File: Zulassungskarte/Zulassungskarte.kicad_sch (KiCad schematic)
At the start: 40 parts, among them J1 Conn_02x04_Counter_Clockwise, J2 Conn_02x04_Counter_Clockwise, J3 Conn_01x04_Pin, J4 Conn_02x03_Odd_Even, U1 ATmega48

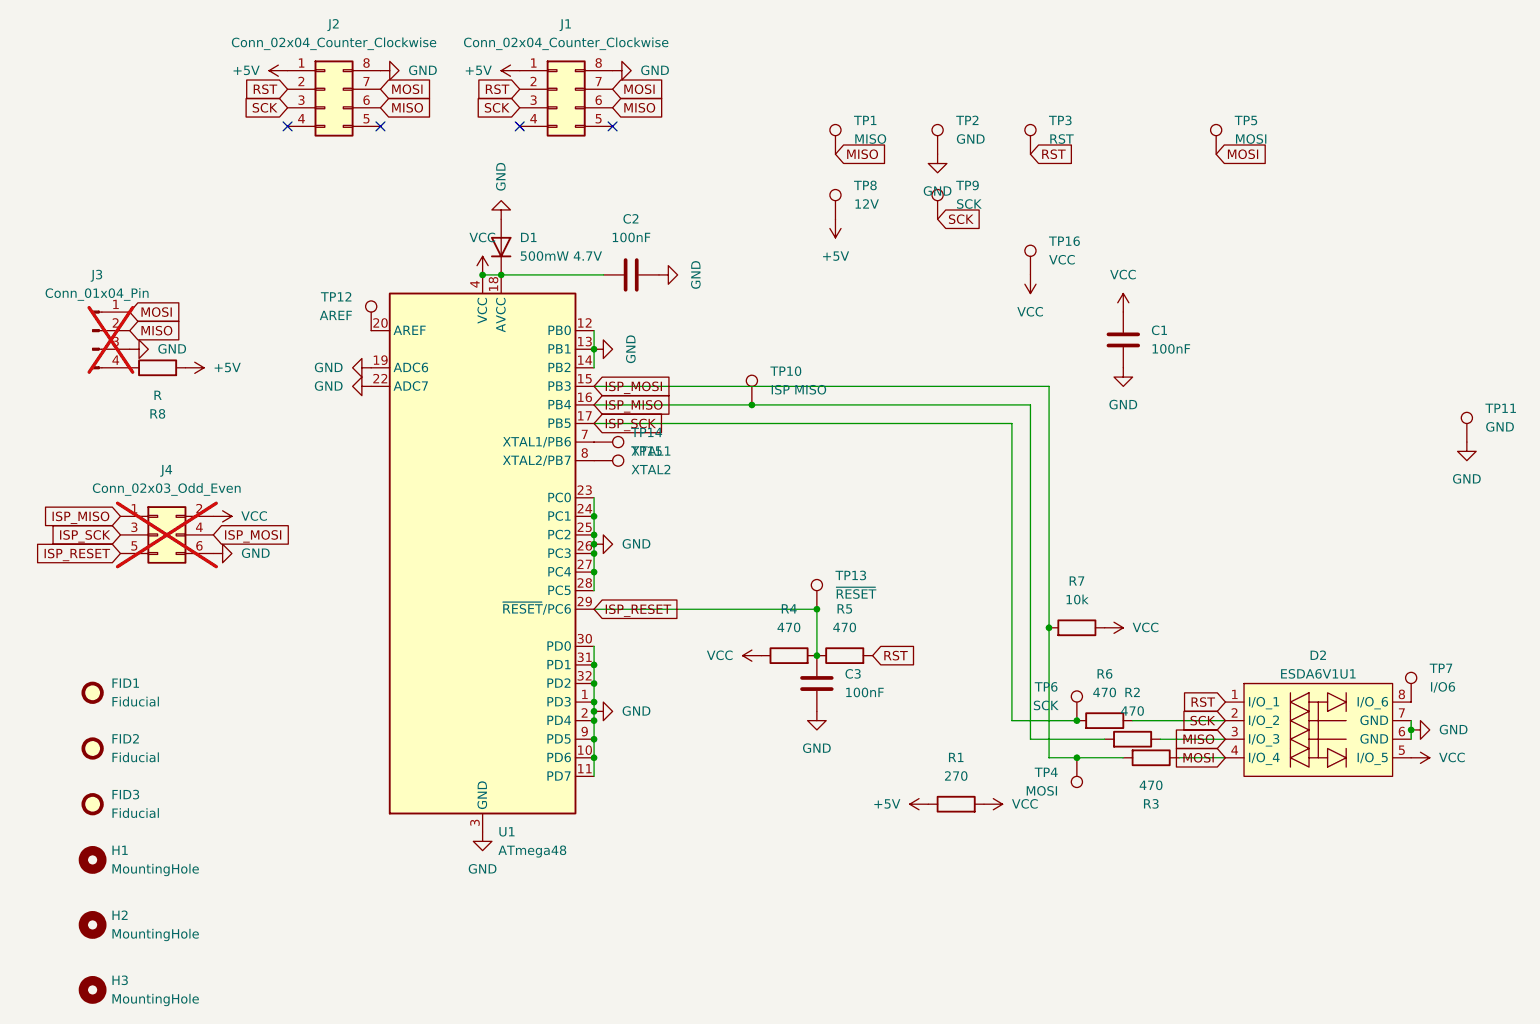
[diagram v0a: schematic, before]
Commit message: 12v zlk
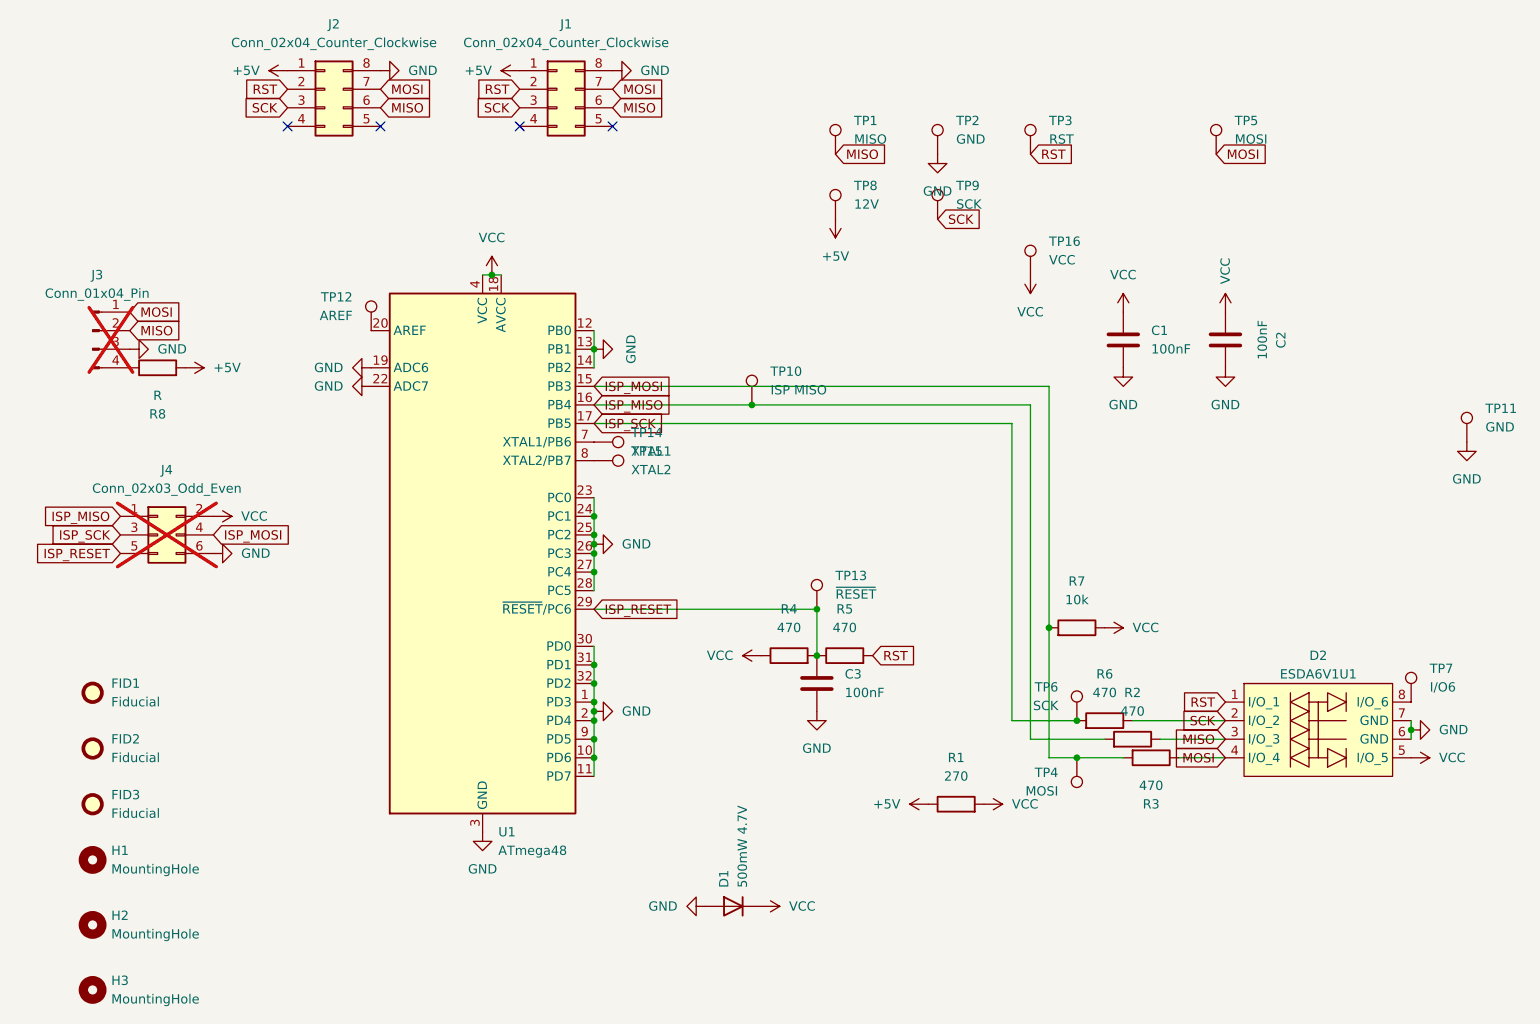
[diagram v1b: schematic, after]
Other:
- moved on the sheet: C2, D1
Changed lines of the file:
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@@
 	)
 	(junction
-		(at 72.39 49.53)
-		(diameter 0)
-		(color 0 0 0 0)
-	)
-	(junction
 		(at 87.63 59.69)
 		(diameter 0)
@@
 	)
 	(junction
-		(at 74.93 49.53)
+		(at 87.63 105.41)
 		(diameter 0)
 		(color 0 0 0 0)
 	)
 	(junction
-		(at 87.63 105.41)
+		(at 87.63 109.22)
 		(diameter 0)
 		(color 0 0 0 0)
 	)
 	(junction
-		(at 87.63 109.22)
+		(at 73.66 49.53)
 		(diameter 0)
 		(color 0 0 0 0)
@@
 	(wire
 		(pts
-			(xy 72.39 49.53) (xy 74.93 49.53)
-		)
-		(stroke
-			(width 0)
-			(type default)
-		)
-	)
-	(wire
-		(pts
 			(xy 157.48 113.03) (xy 147.32 113.03)
 		)
@@
 	(wire
 		(pts
-			(xy 87.63 100.33) (xy 87.63 102.87)
+			(xy 73.66 49.53) (xy 74.93 49.53)
 		)
 		(stroke
@@
 	(wire
 		(pts
-			(xy 87.63 90.17) (xy 87.63 92.71)
+			(xy 87.63 100.33) (xy 87.63 102.87)
 		)
 		(stroke
@@
 	(wire
 		(pts
-			(xy 74.93 49.53) (xy 88.9 49.53)
+			(xy 87.63 90.17) (xy 87.63 92.71)
 		)
 		(stroke
@@
 	(wire
 		(pts
+			(xy 73.66 49.53) (xy 72.39 49.53)
+		)
+		(stroke
+			(width 0)
+			(type default)
+		)
+	)
+	(wire
+		(pts
 			(xy 87.63 107.95) (xy 87.63 105.41)
 		)
@@
 	(symbol
 		(lib_id "power:GND")
-		(at 74.93 41.91 0)
+		(at 102.87 135.89 270)
 		(mirror x)
 		(unit 1)
@@
 		(fields_autoplaced yes)
 		(property "Reference" "#PWR024"
-			(at 74.93 35.56 0)
+			(at 96.52 135.89 0)
 			(effects
 				(font
@@
 		)
 		(property "Value" "GND"
-			(at 74.9301 38.1 90)
+			(at 99.06 135.8899 90)
 			(effects
 				(font
@@
 		)
 		(property "Footprint" ""
-			(at 74.93 41.91 0)
+			(at 102.87 135.89 0)
 			(effects
 				(font
@@
 		)
 		(property "Datasheet" ""
-			(at 74.93 41.91 0)
+			(at 102.87 135.89 0)
 			(effects
 				(font
@@
 		)
 		(property "Description" "Power symbol creates a global label with name \"GND\" , ground"
-			(at 74.93 41.91 0)
+			(at 102.87 135.89 0)
 			(effects
 				(font
@@
 	(symbol
 		(lib_id "power:VCC")
-		(at 72.39 49.53 0)
+		(at 73.66 49.53 0)
 		(unit 1)
 		(exclude_from_sim no)
@@
 		(fields_autoplaced yes)
 		(property "Reference" "#PWR03"
-			(at 72.39 53.34 0)
+			(at 73.66 53.34 0)
 			(effects
 				(font
@@
 		)
 		(property "Value" "VCC"
-			(at 72.39 44.45 0)
+			(at 73.66 44.45 0)
 			(effects
 				(font
@@
 		)
 		(property "Footprint" ""
-			(at 72.39 49.53 0)
+			(at 73.66 49.53 0)
 			(effects
 				(font
@@
 		)
 		(property "Datasheet" ""
-			(at 72.39 49.53 0)
+			(at 73.66 49.53 0)
 			(effects
 				(font
@@
 		)
 		(property "Description" "Power symbol creates a global label with name \"VCC\""
-			(at 72.39 49.53 0)
+			(at 73.66 49.53 0)
 			(effects
 				(font
@@
 	)
 	(symbol
+		(lib_id "power:VCC")
+		(at 110.49 135.89 270)
+		(unit 1)
+		(exclude_from_sim no)
+		(in_bom yes)
+		(on_board yes)
+		(dnp no)
+		(fields_autoplaced yes)
+		(property "Reference" "#PWR08"
+			(at 106.68 135.89 0)
+			(effects
+				(font
+					(size 1.27 1.27)
+				)
+				(hide yes)
+			)
+		)
+		(property "Value" "VCC"
+			(at 114.3 135.8899 90)
+			(effects
+				(font
+					(size 1.27 1.27)
+				)
+				(justify left)
+			)
+		)
+		(property "Footprint" ""
+			(at 110.49 135.89 0)
+			(effects
+				(font
+					(size 1.27 1.27)
+				)
+				(hide yes)
+			)
+		)
+		(property "Datasheet" ""
+			(at 110.49 135.89 0)
+			(effects
+				(font
+					(size 1.27 1.27)
+				)
+				(hide yes)
+			)
+		)
+		(property "Description" "Power symbol creates a global label with name \"VCC\""
+			(at 110.49 135.89 0)
+			(effects
+				(font
+					(size 1.27 1.27)
+				)
+				(hide yes)
+			)
+		)
+		(pin "1"
+		)
+		(instances
+			(project "Zulassungskarte"
+				(path "/f437cf05-d297-460e-8639-991b777c08ac"
+					(reference "#PWR08")
+					(unit 1)
+				)
+			)
+		)
+	)
+	(symbol
 		(lib_id "power:GND")
 		(at 199.39 111.76 90)
@@
 	(symbol
 		(lib_id "Device:D")
-		(at 74.93 45.72 270)
-		(mirror x)
+		(at 106.68 135.89 0)
+		(mirror y)
 		(unit 1)
 		(exclude_from_sim no)
@@
 		(fields_autoplaced yes)
 		(property "Reference" "D1"
-			(at 77.47 44.4499 90)
+			(at 105.4099 133.35 90)
 			(effects
 				(font
@@
 		)
 		(property "Value" "500mW 4.7V"
-			(at 77.47 46.9899 90)
+			(at 107.9499 133.35 90)
 			(effects
 				(font
@@
 		)
 		(property "Footprint" "Diode_SMD:D_SOD-123"
-			(at 74.93 45.72 0)
+			(at 106.68 135.89 0)
 			(effects
 				(font
@@
 		)
 		(property "Datasheet" "~"
-			(at 74.93 45.72 0)
+			(at 106.68 135.89 0)
 			(effects
 				(font
@@
 		)
 		(property "Description" "Diode"
-			(at 74.93 45.72 0)
+			(at 106.68 135.89 0)
 			(effects
 				(font
@@
 		)
 		(property "Sim.Device" "D"
-			(at 74.93 45.72 0)
+			(at 106.68 135.89 0)
 			(effects
 				(font
@@
 		)
 		(property "Sim.Pins" "1=K 2=A"
-			(at 74.93 45.72 0)
+			(at 106.68 135.89 0)
 			(effects
 				(font
@@
 	(symbol
 		(lib_id "Device:C")
-		(at 92.71 49.53 90)
+		(at 173.99 58.42 0)
 		(unit 1)
 		(exclude_from_sim no)
@@
 		(fields_autoplaced yes)
 		(property "Reference" "C2"
-			(at 92.71 41.91 90)
+			(at 181.61 58.42 90)
 			(effects
 				(font
@@
 		)
 		(property "Value" "100nF"
-			(at 92.71 44.45 90)
+			(at 179.07 58.42 90)
 			(effects
 				(font
@@
 		)
 		(property "Footprint" "Capacitor_SMD:C_0805_2012Metric_Pad1.18x1.45mm_HandSolder"
-			(at 96.52 48.5648 0)
+			(at 174.9552 62.23 0)
 			(effects
 				(font
@@
 		)
 		(property "Datasheet" "~"
-			(at 92.71 49.53 0)
+			(at 173.99 58.42 0)
 			(effects
 				(font
@@
 		)
 		(property "Description" "Unpolarized capacitor"
-			(at 92.71 49.53 0)
+			(at 173.99 58.42 0)
 			(effects
 				(font
@@
 	)
 	(symbol
+		(lib_id "power:VCC")
+		(at 173.99 54.61 0)
+		(unit 1)
+		(exclude_from_sim no)
+		(in_bom yes)
+		(on_board yes)
+		(dnp no)
+		(fields_autoplaced yes)
+		(property "Reference" "#PWR019"
+			(at 173.99 58.42 0)
+			(effects
+				(font
+					(size 1.27 1.27)
+				)
+				(hide yes)
+			)
+		)
+		(property "Value" "VCC"
+			(at 173.9901 50.8 90)
+			(effects
+				(font
+					(size 1.27 1.27)
+				)
+				(justify left)
+			)
+		)
+		(property "Footprint" ""
+			(at 173.99 54.61 0)
+			(effects
+				(font
+					(size 1.27 1.27)
+				)
+				(hide yes)
+			)
+		)
+		(property "Datasheet" ""
+			(at 173.99 54.61 0)
+			(effects
+				(font
+					(size 1.27 1.27)
+				)
+				(hide yes)
+			)
+		)
+		(property "Description" "Power symbol creates a global label with name \"VCC\""
+			(at 173.99 54.61 0)
+			(effects
+				(font
+					(size 1.27 1.27)
+				)
+				(hide yes)
+			)
+		)
+		(pin "1"
+		)
+		(instances
+			(project "Zulassungskarte"
+				(path "/f437cf05-d297-460e-8639-991b777c08ac"
+					(reference "#PWR019")
+					(unit 1)
+				)
+			)
+		)
+	)
+	(symbol
 		(lib_id "power:GND")
-		(at 96.52 49.53 90)
+		(at 173.99 62.23 0)
 		(unit 1)
 		(exclude_from_sim no)
@@
 		(fields_autoplaced yes)
 		(property "Reference" "#PWR010"
-			(at 102.87 49.53 0)
+			(at 173.99 68.58 0)
 			(effects
 				(font
@@
 		)
 		(property "Value" "GND"
-			(at 101.6 49.53 0)
+			(at 173.99 67.31 0)
 			(effects
 				(font
@@
 		)
 		(property "Footprint" ""
-			(at 96.52 49.53 0)
+			(at 173.99 62.23 0)
 			(effects
 				(font
@@
 		)
 		(property "Datasheet" ""
-			(at 96.52 49.53 0)
+			(at 173.99 62.23 0)
 			(effects
 				(font
@@
 		)
 		(property "Description" "Power symbol creates a global label with name \"GND\" , ground"
-			(at 96.52 49.53 0)
+			(at 173.99 62.23 0)
 			(effects
 				(font
